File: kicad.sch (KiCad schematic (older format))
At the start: 46 parts, among them J1 Screw_Terminal_01x03, J2 Conn_01x06, J3 Screw_Terminal_01x03, J4 Conn_01x03, J5 Conn_01x03, J6 Conn_01x03, J7 Conn_01x04, J8 Screw_Terminal_01x02, K1 SANYOU_SRD_Form_C, K2 SANYOU_SRD_Form_C, Q1 BC817, Q2 BC817, Q3 BC817, Q4 BC817, Q5 IRF540N, U1 4N25, U2 4N25, U3 4N25, U4 4N25, U5 ACS759xCB-050B-PFF, U6 ESP32_DevKit_V1_DOIT

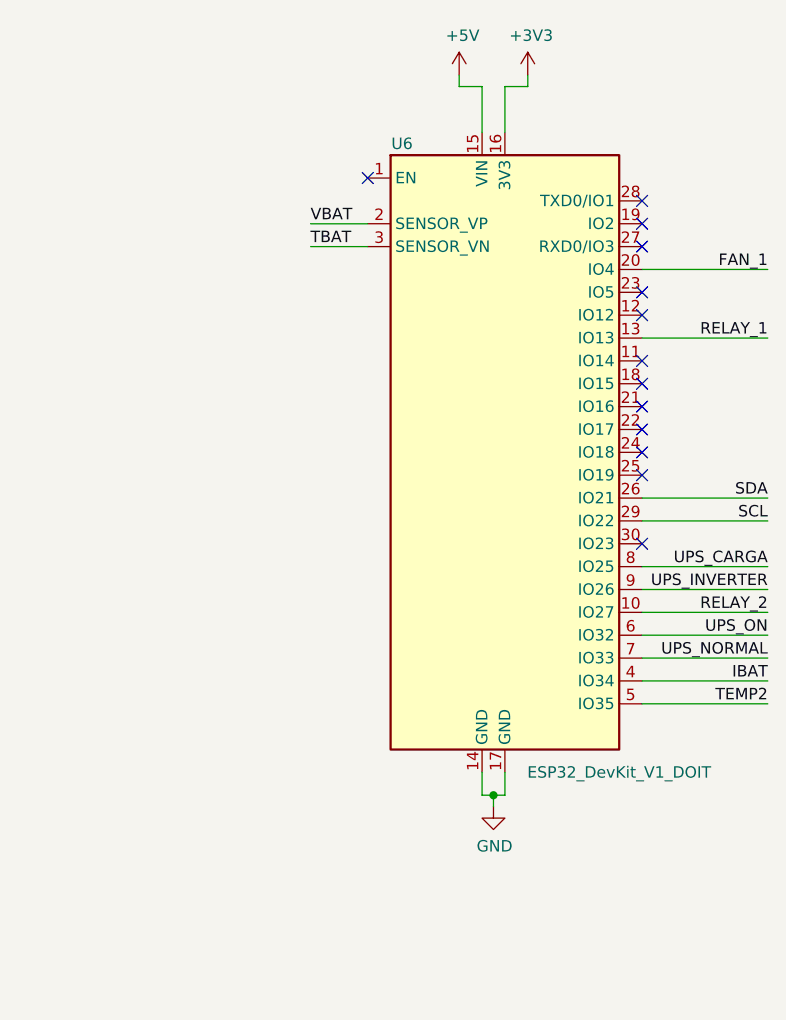
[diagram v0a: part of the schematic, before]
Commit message: update .gitignore
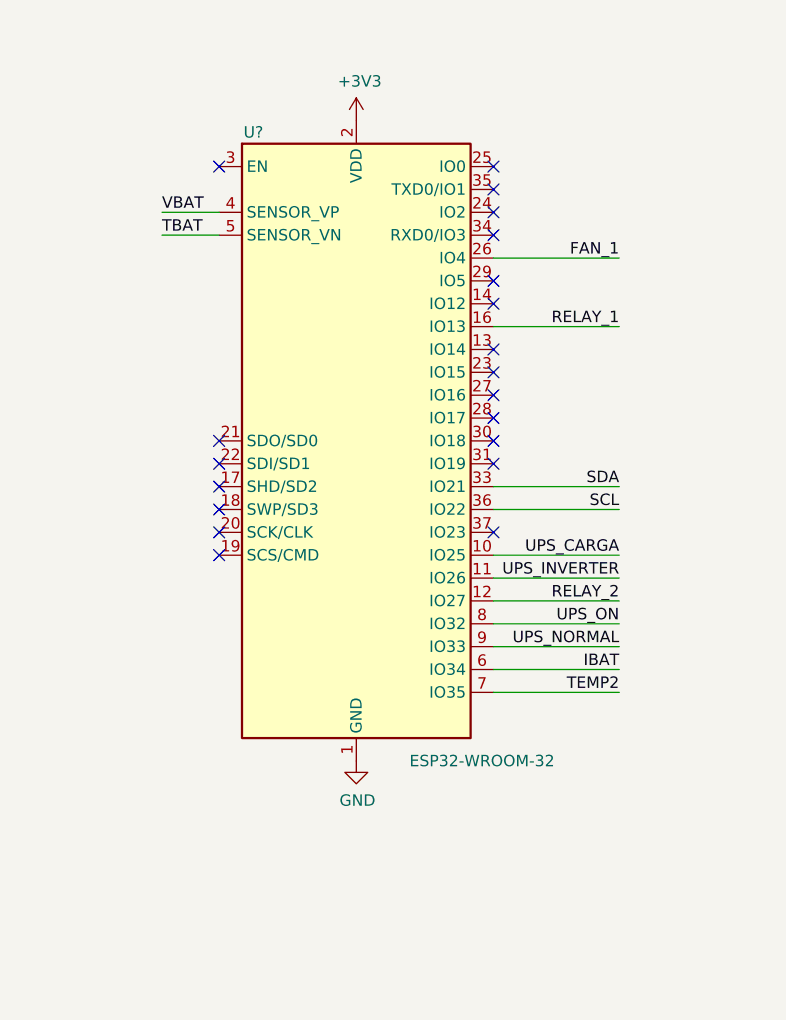
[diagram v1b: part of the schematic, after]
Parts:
- removed U6: ESP32_DevKit_V1_DOIT, ESP32_DevKit_V1_DOIT:esp32_devkit_v1_doit, symbol esp32_devkit_v1_doit:ESP32_DevKit_V1_DOIT
- added U?: ESP32-WROOM-32, RF_Module:ESP32-WROOM-32, symbol RF_Module:ESP32-WROOM-32
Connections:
- net +3V3: now also U?.2 (VDD)
- net FAN_1: now also U?.26 (IO4)
- net GND: now also U?.1 (GND), U?.15 (GND), U?.38 (GND), U?.39 (GND)
- net IBAT: now also U?.6 (IO34)
- net RELAY_1: now also U?.16 (IO13)
- net RELAY_2: now also U?.12 (IO27)
- net SCL: now also U?.36 (IO22)
- net SDA: now also U?.33 (IO21)
- net TBAT: now also U?.5 (SENSOR_VN)
- net TEMP2: now also U?.7 (IO35)
- net UPS_CARGA: now also U?.10 (IO25)
- net UPS_INVERTER: now also U?.11 (IO26)
- net UPS_NORMAL: now also U?.9 (IO33)
- net UPS_ON: now also U?.8 (IO32)
- net VBAT: now also U?.4 (SENSOR_VP)
- no-connect marks 18 -> 25
